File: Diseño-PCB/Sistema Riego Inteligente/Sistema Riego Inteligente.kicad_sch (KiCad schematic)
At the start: 7 parts, among them J1 electroválvula, U1 DEVKIT_V1_ESP32-WROOM-32, U2 DHT11

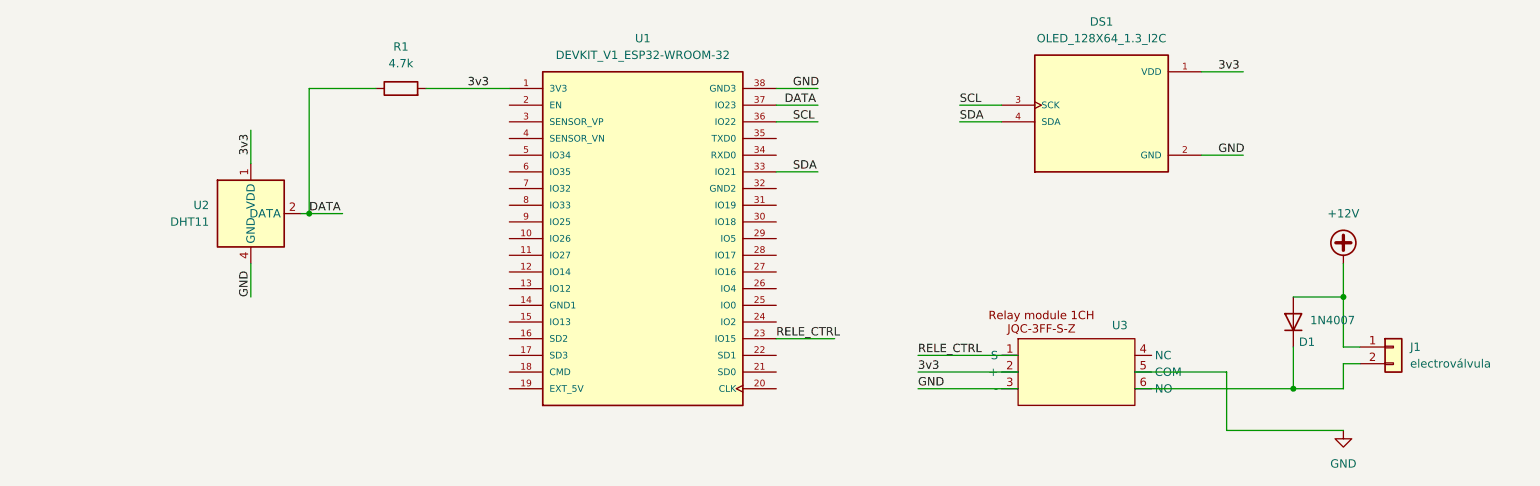
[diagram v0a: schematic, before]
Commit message: Completo ruteo y diseño de PCB
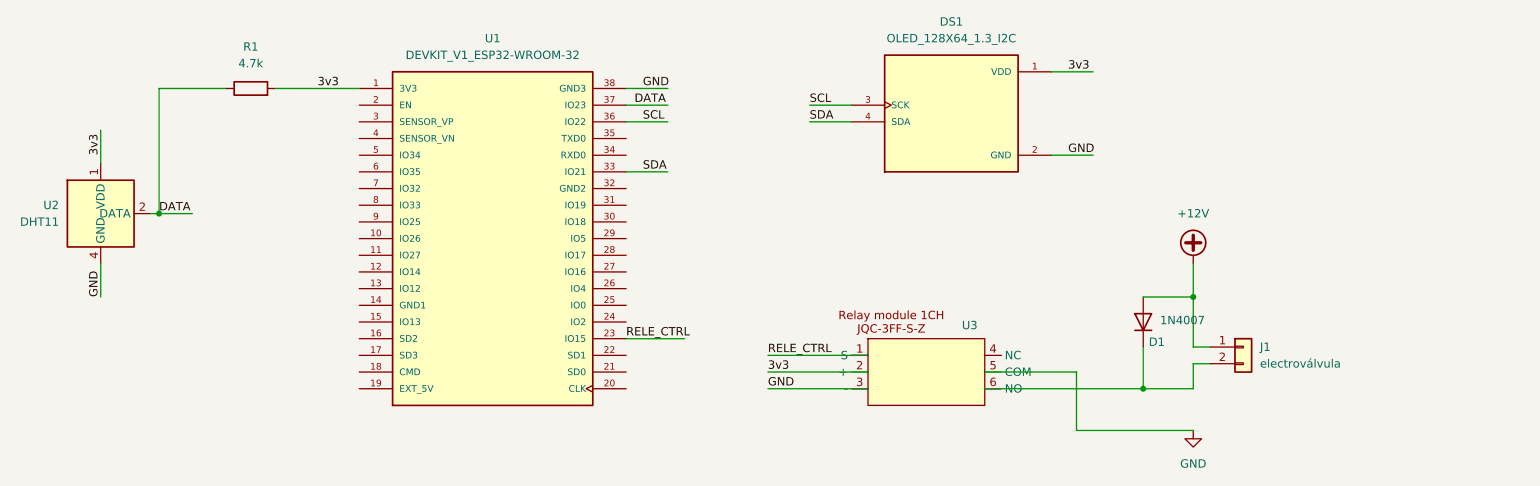
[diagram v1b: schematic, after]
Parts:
- J1: footprint Connector_Phoenix_MC:PhoenixContact_MC_1,5_2-GF-3.5_1x02_P3.50mm_Horizontal_ThreadedFlange -> Connector_Phoenix_GMSTB:PhoenixContact_GMSTBA_2,5_2-G_1x02_P7.50mm_Horizontal
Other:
- moved on the sheet: D1, DS1, J1, R1, U1, U2, U3
